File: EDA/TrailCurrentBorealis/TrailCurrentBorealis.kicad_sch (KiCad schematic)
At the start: 11 parts, among them IC1 SN65HVD230DR, J2 S4B-XH-SM4-TB, U1 ESP32-S3-Zero, U2 GY-SGP30, U3 Mini560, U4 SHT31-D-TempHumidity

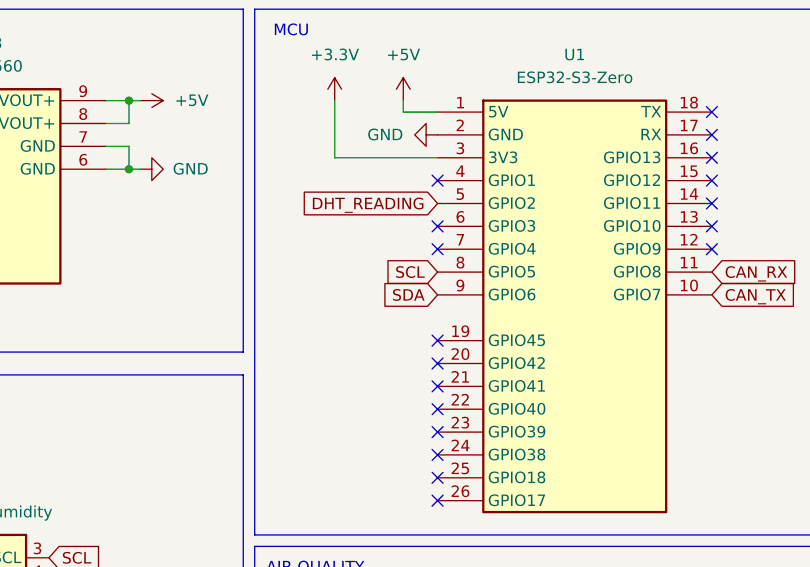
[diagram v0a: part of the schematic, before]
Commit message: Updated PCB for DIY build
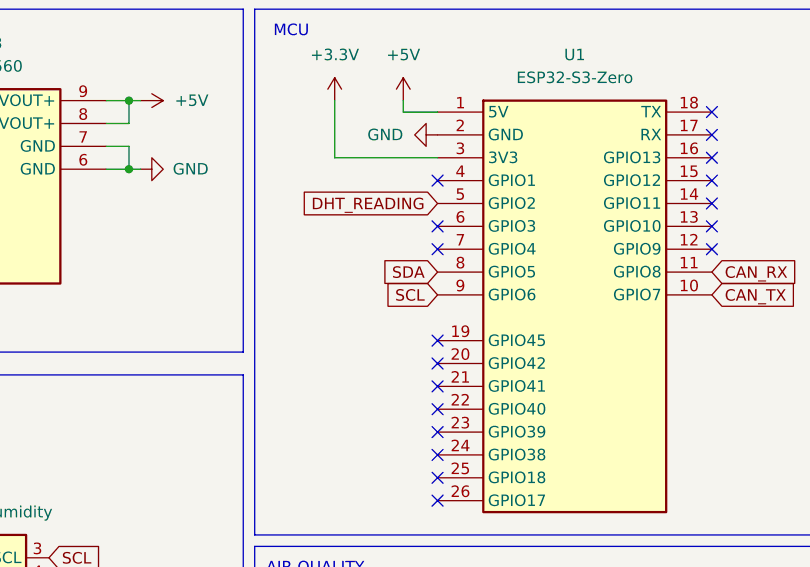
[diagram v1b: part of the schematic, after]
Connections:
- net SCL: now also U1.9 (GPIO6); no longer U1.8 (GPIO5)
- net SDA: now also U1.8 (GPIO5); no longer U1.9 (GPIO6)
